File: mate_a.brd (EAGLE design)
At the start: 92.7 x 100 mm, 8 parts, among them IC1 PIC18F47Q84-E_P, X1 GLX-S-88M

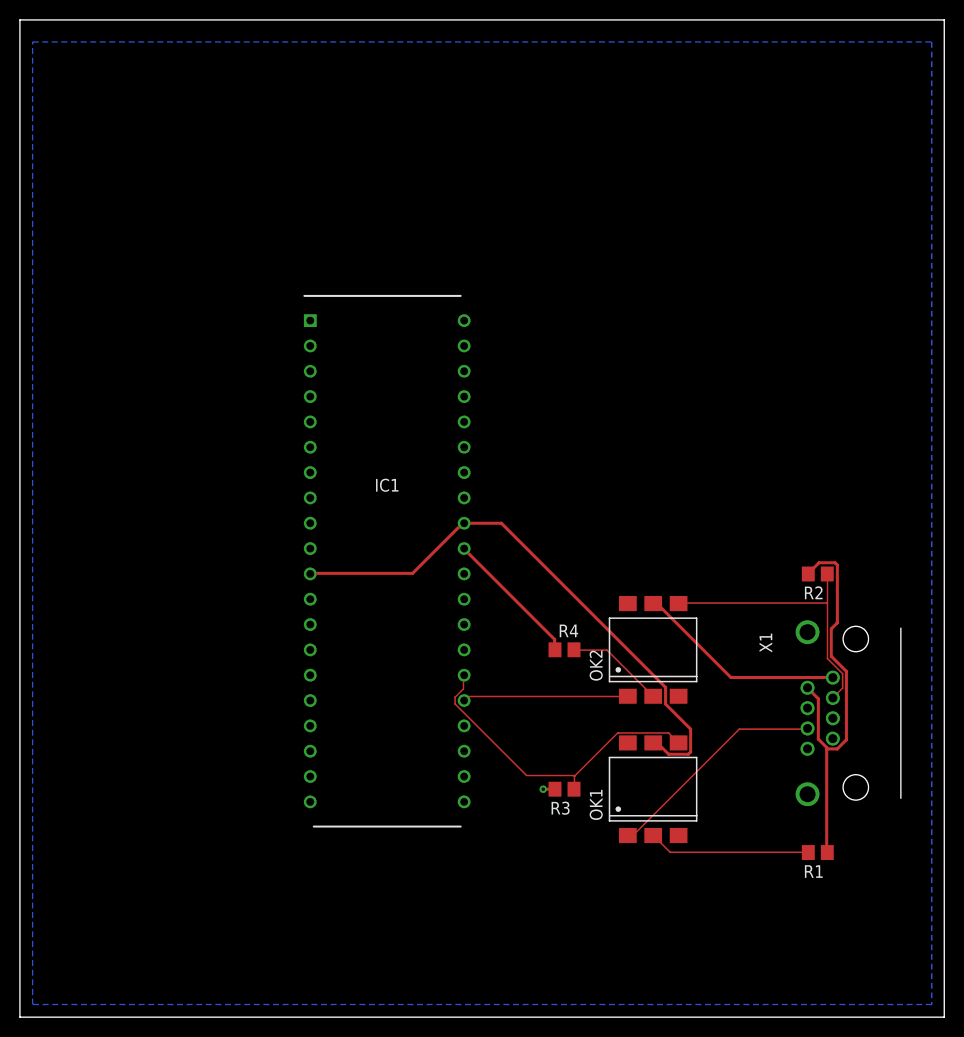
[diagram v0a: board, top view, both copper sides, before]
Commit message: up
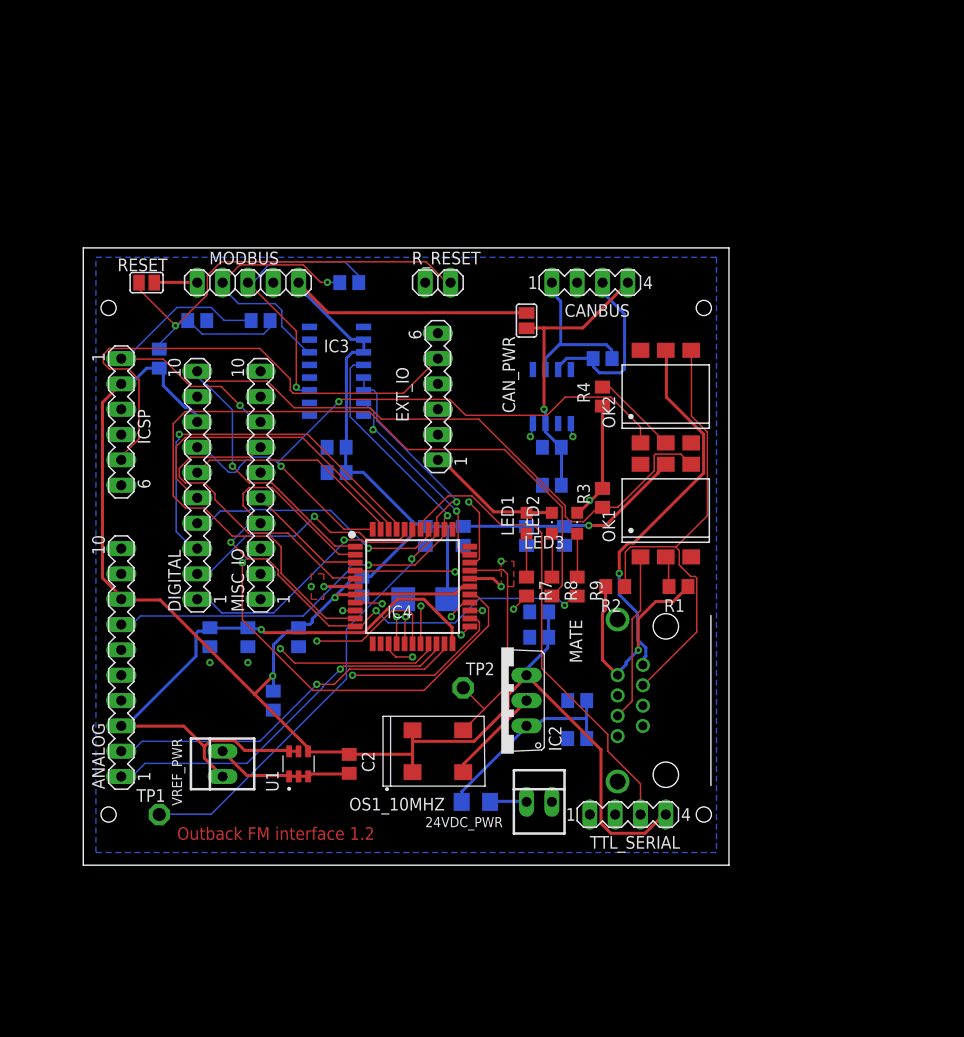
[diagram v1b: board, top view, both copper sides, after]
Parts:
- removed IC1: PIC18F47Q84-E_P, PIC18F47Q84-E_P:DIP1543W58P254L5175H635Q40N
- removed X1: GLX-S-88M, con-kycon:GLX-S-88M
- added 24VDC_PWR: 24vdc power, con-molex:22-23-2021
- added ANALOG: Analog, con-lstb:MA10-1
- added C1, C11, C12, C14, C16, C18, C2, C3, C5, C7, C9: 0.1uf, rcl:C0805
- added C10, C13, C15, C17, C19, C4, C6, C8: 10uf, rcl:C0805
- added CANBUS: CANBUS, con-lstb:MA04-1
- added CAN_PWR: CAN_PWR, jumper:SJ
- added DIGITAL: Digtal, con-lstb:MA10-1
- added EXT_IO: EXT_IO, con-lstb:MA06-1
- added IC2: 7805TV, linear:TO220V
- added IC3: ADM3095EBRZ, ADM3095EBRZ:SOIC127P600X175-16N
- added IC4: PIC18F47Q84-I_PT, PIC18F47Q84-I_PT:QFP80P1200X1200X120-44N
- added ICSP: ICSP, con-lstb:MA06-1
- added LED1: run, led:CHIPLED_0805
- added LED2: error, led:CHIPLED_0805
- added LED3: comm, led:CHIPLED_0805
- added MATE: GLX-S-88M, con-kycon:GLX-S-88M
- added MISC_IO: misc-io, con-lstb:MA10-1
- added MODBUS: MODBUS, pinhead:1X05
- added OS1_10MHZ: OSC-OE-CFPS-72, IQD-Frequency-Products:7.2X5.2-4-PAD
- added R10: 120ohm, rcl:R0805
- added R11: 120, rcl:R0805
- added R12: 0 ohm fuse, rcl:R1206
- added R5: 56ohm, rcl:R0805
- added R6: 10k, rcl:R0805
- added R7, R8, R9: 1k, rcl:R0805
- added RESET: reset, jumper:SJ
- added R_RESET: remote_reset, pinhead:1X02
- added TP1, TP2: PTR1PAD1-13, testpad:P1-13
- added TTL_SERIAL: TTL Serial, con-lstb:MA04-1
- added U1: REF3440IDBVR, REF3440IDBVR:SOT95P280X145-6N
- added U2: TCAN330GDR, TCAN330GDR:SOIC127P600X175-8N
- added VREF_PWR: 5vdc_vref_pwr, con-molex:22-23-2021
- added ZENER: 5.6V, diode:SMB
- R1, R2: value (none) -> 2.2k
- R3: value (none) -> 1k
- R4: value (none) -> 470ohm
- moved R1 30.1 mm to (133.3, 43.2)
- moved R3 29.5 mm to (125.7, 52.1), turned to 90 degrees
- moved OK1 28.0 mm to (132.1, 50.8)
- moved R4 25.7 mm to (125.7, 62.2), turned to 90 degrees
- moved OK2 25.4 mm to (132.1, 62.2)
- moved R2 20.4 mm to (127.0, 43.2)
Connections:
- removed net PC_RX: IC1.26, OK1.4, R3.1
- removed net PC_TX: IC1.25, OK2.1
- new net AN0: ANALOG.10, IC4.19
- new net AN1: ANALOG.1, IC4.20
- new net AN2: ANALOG.2, IC4.21
- new net AN4: ANALOG.4, IC4.23
- new net AN5: ANALOG.5, IC4.24
- new net CANRX: IC4.8, U2.4
- new net CANTX: IC4.14, U2.1
- new net CAN_N: CANBUS.1, R10.1, U2.6
- new net CAN_P: CANBUS.3, R10.2, U2.7
- new net CAN_VCC: C7.1, C8.1, CANBUS.4, CAN_PWR.1, U2.3
- new net CLOCKO: IC4.31, MISC_IO.10
- new net CPU_CLK: IC4.30, OS1_10MHZ.3, TP2.TP
- new net CS: DIGITAL.3, IC4.41
- new net DB0: DIGITAL.1, IC4.39
- new net DB1: DIGITAL.2, IC4.40
- new net DERE: IC3.5, IC3.6, IC4.36, TP1.TP
- new net DLED: IC4.11, IC4.2, MISC_IO.4, R9.2
- new net MB_A: IC3.11, MODBUS.3, R11.1
- new net MB_B: IC3.14, MODBUS.2, R11.2
- new net MB_RX: ANALOG.6, IC3.7, IC4.32
- new net MB_TX: ANALOG.7, IC3.4, IC4.35
- new net MCLR_SIG: IC4.18, ICSP.1, MISC_IO.8, R5.2
- new net MISC: IC4.26, MISC_IO.2
- new net MLED: IC4.9, R7.2
- new net N$2: C14.1, C15.1, IC2.1, R12.1
- new net N$4: LED1.A, R7.1
- new net N$5: LED2.A, R8.1
- new net N$6: LED3.A, R9.1
- new net PC_RX2: IC4.38, TTL_SERIAL.3
- new net PC_TX2: IC4.4, TTL_SERIAL.2
- new net PGC: EXT_IO.5, IC4.16, ICSP.5
- new net PGD: EXT_IO.6, IC4.17, ICSP.4
- new net RB5: EXT_IO.4, IC4.15, MISC_IO.6
- new net RD5: EXT_IO.2, IC4.3, MISC_IO.5
- new net RD7: EXT_IO.3, IC4.5, MISC_IO.7
- new net RE2: IC4.27, MISC_IO.3
- new net RELAY: IC4.25, MISC_IO.1
- new net RLED: IC4.10, R8.2
- new net R_RESET: C1.1, R5.1, R6.1, RESET.1, R_RESET.2
- new net SCK1: DIGITAL.4, IC4.37
- new net SDI1: DIGITAL.5, IC4.42
- new net SDO1: DIGITAL.6, IC4.43
- new net UC_RX: DIGITAL.10, IC4.1, OK1.4, R3.1
- new net UC_TX: DIGITAL.7, IC4.44, OK2.1
- new net V+: 24VDC_PWR.1, R12.2
- new net VREF: ANALOG.3, C16.1, C17.1, IC4.22, U1.5, U1.6, VREF_PWR.1
- net +24V: now also MATE.1; no longer X1.1
- net 0V: now also MATE.2; no longer X1.2
- net MX_RX: now also MATE.6; no longer X1.6
- net MX_TX: now also MATE.3; no longer X1.3
- net VDD: now also ANALOG.8, C10.1, C11.1, C12.1, C13.1, C18.1, C19.1, C2.1, C3.1, C4.1, C5.1, C6.1, C9.1, CAN_PWR.2, DIGITAL.8, IC2.3, IC3.2, IC3.3, IC4.28, IC4.7, ICSP.2, MODBUS.5, OS1_10MHZ.1, OS1_10MHZ.4, R6.2, TTL_SERIAL.4, U1.4, ZENER.C; no longer IC1.11, IC1.32
- net VSS: now also 24VDC_PWR.2, ANALOG.9, C1.2, C10.2, C11.2, C12.2, C13.2, C14.2, C15.2, C16.2, C17.2, C18.2, C19.2, C2.2, C3.2, C4.2, C5.2, C6.2, C7.2, C8.2, C9.2, CANBUS.2, DIGITAL.9, EXT_IO.1, IC2.2, IC3.1, IC3.10, IC3.12, IC3.13, IC3.15, IC3.16, IC3.8, IC3.9, IC4.29, IC4.6, ICSP.3, LED1.C, LED2.C, LED3.C, MISC_IO.9, MODBUS.1, MODBUS.4, OS1_10MHZ.2, RESET.2, R_RESET.1, TTL_SERIAL.1, U1.1, U1.2, U1.3, U2.2, U2.5, U2.8, VREF_PWR.2, ZENER.A; no longer IC1.12, IC1.31
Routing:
- net VDD: track 56.4 -> 256.8 mm, vias 0 -> 3
- net UC_RX: track 0.00 -> 87.3 mm, vias 0 -> 1
- net RLED: track 0.00 -> 85.0 mm
- net PGC: track 0.00 -> 82.5 mm, vias 0 -> 1
- net PGD: track 0.00 -> 80.3 mm, vias 0 -> 1
- net VREF: track 0.00 -> 66.1 mm, vias 0 -> 1
- net MCLR_SIG: track 0.00 -> 66.0 mm, vias 0 -> 2
- net UC_TX: track 0.00 -> 65.6 mm, vias 0 -> 2
- net DERE: track 0.00 -> 64.0 mm, vias 0 -> 2
- net DLED: track 0.00 -> 63.2 mm, vias 0 -> 3
- net MB_TX: track 0.00 -> 58.7 mm, vias 0 -> 2
- net MB_RX: track 0.00 -> 58.0 mm, vias 0 -> 2
- net R_RESET: track 0.00 -> 52.4 mm, vias 0 -> 1
- net RD7: track 0.00 -> 51.5 mm
- net PC_RX2: track 0.00 -> 47.8 mm
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- added copper zone on layer 1, net VSS
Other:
- board size 92.7 x 100 mm -> 64.8 x 61.9 mm
- board text added: "Outback FM interface 1.2"

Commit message: up
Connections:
- net RD5 renamed AUX_RELAY
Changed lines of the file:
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@@
 <via x="102.2604" y="45.339" extent="1-16" drill="0.35"/>
 </signal>
-<signal name="RD5">
+<signal name="AUX_RELAY">
 <contactref element="MISC_IO" pad="5"/>
 <contactref element="IC4" pad="3"/>
